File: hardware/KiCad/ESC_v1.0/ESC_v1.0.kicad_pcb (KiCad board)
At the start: 2 copper layers, 108 parts, among them J3 Conn_ARM_SWD_TagConnect_TC203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, Q1 NVMFS5C604N, Q2 NVMFS5C604N, Q3 NVMFS5C604N, Q4 NVMFS5C604N, Q5 NVMFS5C604N, Q6 NVMFS5C604N, U1 STM32G484CEU6, U2 LM5160A, U3 TPS7B92033, U4 2EDL8024, U5 2EDL8024, U6 2EDL8024, X1 16MHz

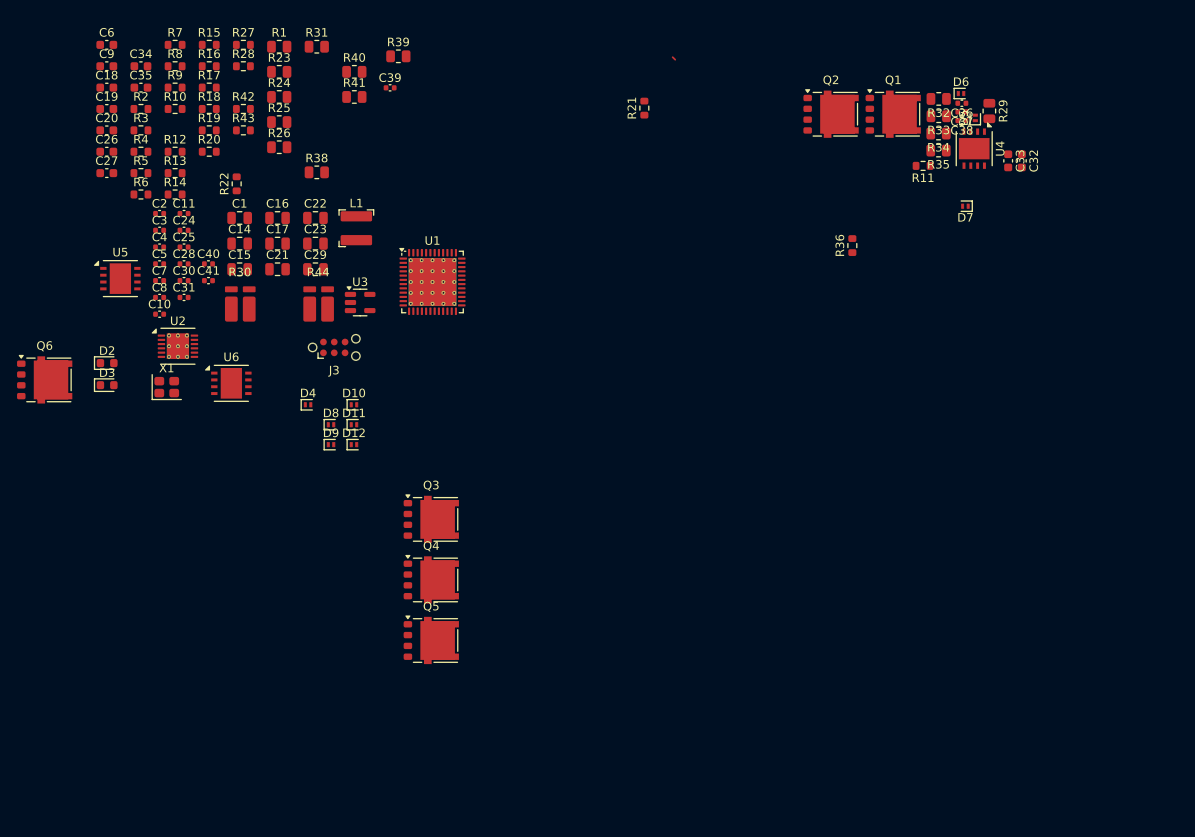
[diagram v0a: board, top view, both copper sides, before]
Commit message: Kicad
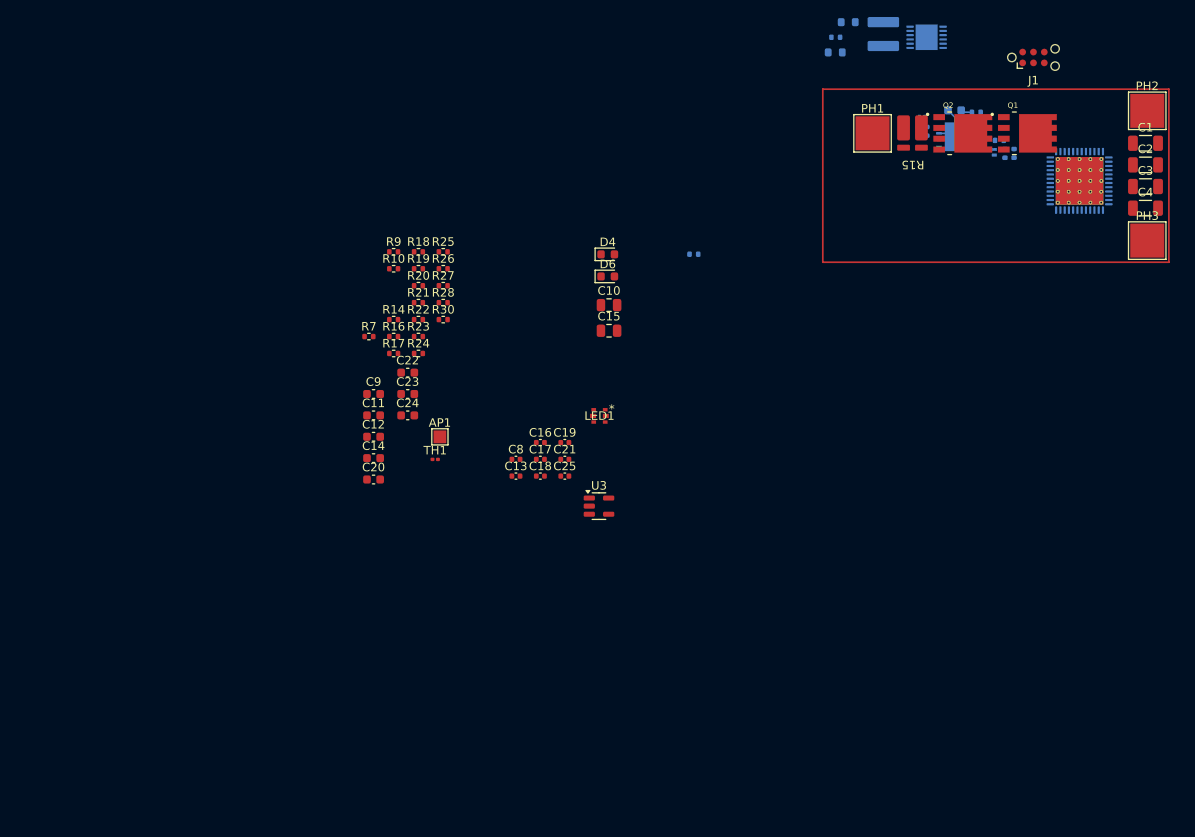
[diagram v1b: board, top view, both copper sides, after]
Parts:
- removed C26, C27, C32, C33, C34, C35: 1u, Capacitor_SMD:C_0603_1608Metric
- removed C28, C30, C31, C36, C37, C38, C39, C40, C41, C7: 100n, Capacitor_SMD:C_0402_1005Metric
- removed C29: 4.7u, Capacitor_SMD:C_0805_2012Metric
- removed D10, D11, D12, D7, D8, D9: RB161QS-40T18R, ESC-FootprintLib:Rohm_SMD1006
- removed J3: Conn_ARM_SWD_TagConnect_TC2030-NL, Connector:Tag-Connect_TC2030-IDC-NL_2x03_P1.27mm_Vertical
- removed Q3, Q4, Q5, Q6: NVMFS5C604N, ESC-FootprintLib:Onsemi_DFN5_DFNW5
- removed R29, R31: 5.1, Resistor_SMD:R_0805_2012Metric
- removed R32, R33, R34, R35, R38, R39, R40, R41: 10, Resistor_SMD:R_0805_2012Metric
- removed R36, R42, R43: 10k, Resistor_SMD:R_0603_1608Metric
- removed R44: 0.5, ESC-FootprintLib:Kelvin Shunt 1216 (3038)
- removed U5, U6: 2EDL8024, Package_DFN_QFN:DFN-8-1EP_4x4mm_P0.8mm_EP2.5x3.6mm
- removed X1: 16MHz, Crystal:Crystal_SMD_2520-4Pin_2.5x2.0mm
- added AP1: ActionPad, TestPoint:TestPoint_Pad_1.5x1.5mm, F.Cu at (68.1, 63.7)
- added C12: 1u, Capacitor_SMD:C_0603_1608Metric, F.Cu at (60.3, 63.7)
- added C13: 10n, Capacitor_SMD:C_0402_1005Metric, F.Cu at (77.0, 68.3)
- added J1: Conn_ARM_SWD_TagConnect_TC2030-NL, Connector:Tag-Connect_TC2030-IDC-NL_2x03_P1.27mm_Vertical, F.Cu at (137.8, 19.1)
- added LED1: 19-337C/RSBHGHC-A88/4T, ESC-FootprintLib:SMD-B_19-337C_EVE, F.Cu at (86.8, 61.2)
- added PH1: ~, TestPoint:TestPoint_Pad_4.0x4.0mm, F.Cu at (118.9, 28.0)
- added PH2: ~, TestPoint:TestPoint_Pad_4.0x4.0mm, F.Cu at (151.1, 25.4)
- added PH3: ~, TestPoint:TestPoint_Pad_4.0x4.0mm, F.Cu at (151.1, 40.6)
- added TH1: Thermistor_NTC, Resistor_SMD:R_0201_0603Metric, F.Cu at (67.5, 66.3)
- C1: value 4.7u -> 2.2u; footprint Capacitor_SMD:C_0805_2012Metric -> Capacitor_SMD:C_1206_3216Metric
- C10: value 10p -> 4.7u; footprint Capacitor_SMD:C_0402_1005Metric -> Capacitor_SMD:C_0805_2012Metric
- C11: value 10p -> 1u; footprint Capacitor_SMD:C_0402_1005Metric -> Capacitor_SMD:C_0603_1608Metric
- C14: value 22u -> 1u; footprint Capacitor_SMD:C_0805_2012Metric -> Capacitor_SMD:C_0603_1608Metric
- C15: value 22u -> 4.7u
- C16, C17: value 22u -> 100n; footprint Capacitor_SMD:C_0805_2012Metric -> Capacitor_SMD:C_0402_1005Metric
- C18, C19: value 1u -> 100n; footprint Capacitor_SMD:C_0603_1608Metric -> Capacitor_SMD:C_0402_1005Metric
- C2, C3, C4: value 100n -> 2.2u; footprint Capacitor_SMD:C_0402_1005Metric -> Capacitor_SMD:C_1206_3216Metric
- C21: value 100p -> 100n; footprint Capacitor_SMD:C_0805_2012Metric -> Capacitor_SMD:C_0402_1005Metric
- C22, C23: footprint Capacitor_SMD:C_0805_2012Metric -> Capacitor_SMD:C_0603_1608Metric
- C24: value 100n -> 100p; footprint Capacitor_SMD:C_0402_1005Metric -> Capacitor_SMD:C_0603_1608Metric
- C25: value 10n -> 100n
- C5: value 10n -> 1u; footprint Capacitor_SMD:C_0402_1005Metric -> Capacitor_SMD:C_0603_1608Metric; moved to B.Cu
- C6: value 1u -> 220n; footprint Capacitor_SMD:C_0603_1608Metric -> Capacitor_SMD:C_0402_1005Metric; moved to B.Cu
- C8: value 100n -> 10n
- D2, D3: value KT-0603W -> RB161QS-40T18R; footprint LED_SMD:LED_0603_1608Metric -> ESC-FootprintLib:Rohm_SMD1006; moved to B.Cu
- D4, D6: value RB161QS-40T18R -> KT-0603W; footprint ESC-FootprintLib:Rohm_SMD1006 -> LED_SMD:LED_0603_1608Metric
- D5, L1, R5: moved to B.Cu
- Q1, Q2: value NVMFS5C604N -> CSD18540Q5B; footprint ESC-FootprintLib:Onsemi_DFN5_DFNW5 -> ESC-FootprintLib:TRANS_CSD18540Q5B
- R1: value 5.1 -> 3.3; footprint Resistor_SMD:R_0805_2012Metric -> Resistor_SMD:R_0402_1005Metric; moved to B.Cu
- R10: value 47 -> 1k; footprint Resistor_SMD:R_0603_1608Metric -> Resistor_SMD:R_0402_1005Metric
- R11: value 10k -> 10; footprint Resistor_SMD:R_0603_1608Metric -> Resistor_SMD:R_0402_1005Metric; moved to B.Cu
- R12: value 47 -> 22k; moved to B.Cu
- R13: value 390 -> 10k; footprint Resistor_SMD:R_0603_1608Metric -> Resistor_SMD:R_0402_1005Metric; moved to B.Cu
- R14: value 390 -> 12k; footprint Resistor_SMD:R_0603_1608Metric -> Resistor_SMD:R_0402_1005Metric
- R15: value 5.6k -> 0.5; footprint Resistor_SMD:R_0603_1608Metric -> ESC-FootprintLib:Kelvin Shunt 1216 (3038)
- R16, R17: value 150 -> 10k; footprint Resistor_SMD:R_0603_1608Metric -> Resistor_SMD:R_0402_1005Metric
- R18: value 150 -> 100; footprint Resistor_SMD:R_0603_1608Metric -> Resistor_SMD:R_0402_1005Metric
- R19, R27, R28: value 10k -> 100; footprint Resistor_SMD:R_0603_1608Metric -> Resistor_SMD:R_0402_1005Metric
- R2: value 390 -> 10; footprint Resistor_SMD:R_0603_1608Metric -> Resistor_SMD:R_0402_1005Metric; moved to B.Cu
- R20: value 39k -> 200k; footprint Resistor_SMD:R_0603_1608Metric -> Resistor_SMD:R_0402_1005Metric
- R21: value 1k -> 33; footprint Resistor_SMD:R_0603_1608Metric -> Resistor_SMD:R_0402_1005Metric
- R22: value 120k -> 33; footprint Resistor_SMD:R_0603_1608Metric -> Resistor_SMD:R_0402_1005Metric
- R23, R25, R26: value 10 -> 1k; footprint Resistor_SMD:R_0805_2012Metric -> Resistor_SMD:R_0402_1005Metric
- R24: value 10 -> 33; footprint Resistor_SMD:R_0805_2012Metric -> Resistor_SMD:R_0402_1005Metric
- R3: value 22k -> 3.3; footprint Resistor_SMD:R_0603_1608Metric -> Resistor_SMD:R_0402_1005Metric; moved to B.Cu
- R30: value 0.5 -> 10k; footprint ESC-FootprintLib:Kelvin Shunt 1216 (3038) -> Resistor_SMD:R_0402_1005Metric
- R4: value 200k -> 10k; footprint Resistor_SMD:R_0603_1608Metric -> Resistor_SMD:R_0402_1005Metric; moved to B.Cu
- R6: value 5.6k -> 200k; footprint Resistor_SMD:R_0603_1608Metric -> Resistor_SMD:R_0402_1005Metric; moved to B.Cu
- R7: value 5.6k -> 100; footprint Resistor_SMD:R_0603_1608Metric -> Resistor_SMD:R_0402_1005Metric
- R8: value 390 -> 3.3; footprint Resistor_SMD:R_0603_1608Metric -> Resistor_SMD:R_0402_1005Metric; moved to B.Cu
- R9: value 47 -> 51k; footprint Resistor_SMD:R_0603_1608Metric -> Resistor_SMD:R_0402_1005Metric
- U1: value STM32G484CEU6 -> 2EDL8024; footprint Package_DFN_QFN:QFN-48-1EP_7x7mm_P0.5mm_EP5.6x5.6mm_ThermalVias -> ESC-FootprintLib:2EDL8x2x_PG-VDSON-8-4; moved to B.Cu
- U2: footprint Package_SON:WSON-12-1EP_4x4mm_P0.5mm_EP2.6x3mm_ThermalVias -> Package_SON:WSON-12-1EP_4x4mm_P0.5mm_EP2.6x3mm; moved to B.Cu
- U4: value 2EDL8024 -> STM32G484CEU6; footprint Package_DFN_QFN:DFN-8-1EP_4x4mm_P0.8mm_EP2.5x3.6mm -> Package_DFN_QFN:QFN-48-1EP_7x7mm_P0.5mm_EP5.6x5.6mm_ThermalVias; moved to B.Cu
- moved C2 115.9 mm to (150.9, 31.8)
- moved C3 115.9 mm to (150.9, 34.3)
- moved C4 115.9 mm to (150.9, 36.8)
- moved D3 107.7 mm to (133.2, 30.3), turned to -90 degrees
- moved D2 106.8 mm to (132.0, 27.0), turned to 90 degrees
- moved C1 106.7 mm to (150.9, 29.2)
- moved C6 103.6 mm to (132.0, 28.8), turned to -90 degrees
- moved R4 102.5 mm to (135.5, 30.4), turned to -90 degrees
- moved R2 101.6 mm to (134.4, 30.4), turned to 90 degrees
- moved U2 95.1 mm to (125.2, 16.8), turned to 180 degrees
- moved C5 95.1 mm to (128.5, 25.3), turned to 180 degrees
- moved R8 94.2 mm to (131.1, 25.6)
- moved R3 92.3 mm to (125.2, 27.8), turned to -90 degrees
- moved R1 85.3 mm to (133.8, 28.9)
- moved R15 84.5 mm to (124.6, 29.7), turned to 180 degrees
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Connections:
- C1 pad 1: +3V3 -> VM
- C1 pad 2: AGND -> PGND
- C10 pad 1: /HSE_OUT -> +3V3
- C10 pad 2: AGND -> GND
- C11 pad 1: /HSE_IN -> Net-(U2-SS)
- C11 pad 2: AGND -> GND
- C14 pad 1: VM -> +3V3A
- C14 pad 2: PGND -> AGND
- C15 pad 1: VM -> +3V3
- C15 pad 2: PGND -> GND
- C16 pad 1: VM -> +3V3
- C16 pad 2: PGND -> GND
- C17 pad 1: VM -> +3V3
- C17 pad 2: PGND -> GND
- C18 pad 1: +10V -> +3V3
- C18 pad 2: AGND -> GND
- C19 pad 1: Net-(U2-SS) -> +3V3REF
- C2 pad 1: +3V3 -> VM
- C2 pad 2: AGND -> PGND
- C20 pad 1: Net-(U2-FPWM) -> +3V3REF
- C21 pad 1: Net-(C21-Pad1) -> +3.3V
- C21 pad 2: AGND -> GND
- C22 pad 1: Net-(C22-Pad1) -> VSENSE1
- C22 pad 2: AGND -> GND
- C23 pad 1: Net-(C23-Pad1) -> VSENSE2
- C23 pad 2: AGND -> GND
- C24 pad 1: +3.3V -> VSENSE3
- C24 pad 2: AGND -> GND
- C25 pad 1: +10VNoise -> DEBUG_NRST
- C25 pad 2: Net-(U2-BST) -> GND
- C3 pad 1: +3V3 -> VM
- C3 pad 2: AGND -> PGND
- C4 pad 1: +3V3 -> VM
- C4 pad 2: AGND -> PGND
- C5 pad 1: +3V3A -> +10V
- C5 pad 2: AGND -> GND
- C6 pad 1: +3V3A -> /HB1
- C6 pad 2: AGND -> PH1
- C8 pad 1: DEBUG_NRST -> +10.5VNoise
- C8 pad 2: AGND -> Net-(U2-BST)
- C9 pad 1: +3V3REF -> +10.5V
- C9 pad 2: AGND -> GND
- D2 pad 1: AGND -> /HB1
- D3 pad 1: AGND -> /HO
- D4 pad 1: Net-(D4-K) -> GND
- D5 pad 1: /HB1 -> /LO
- D6 pad 1: /HO1 -> GND
- L1 pad 1: +10VNoise -> +10.5VNoise
- L1 pad 2: +10V -> +10.5V
- R1 pad 1: +10V -> /HO
- R1 pad 2: Net-(D4-A) -> Net-(Q1-G)
- R10 pad 1: VSENSE2 -> +10.5V
- R10 pad 2: Net-(C22-Pad1) -> Net-(D6-A)
- R11 pad 1: Net-(Q2-G) -> Net-(D5-A)
- R11 pad 2: AGND -> Net-(Q2-G)
- R12 pad 1: VSENSE3 -> Net-(U2-EN/UVLO)
- R12 pad 2: Net-(C23-Pad1) -> GND
- R13 pad 1: VSENSE2 -> Net-(Q2-G)
- R13 pad 2: AGND -> GND
- R14 pad 1: VSENSE1 -> Net-(U2-FB)
- R14 pad 2: AGND -> GND
- R15 pad 1: PH3 -> ISENSE1
- R15 pad 2: VSENSE3 -> GPH1
- R16 pad 1: +3V3 -> Net-(R16-Pad1)
- R16 pad 2: Net-(D3-A) -> PH1
- R17 pad 1: RGB_LED_G -> Net-(R17-Pad1)
- R17 pad 2: /LED_G_K -> PH2
- R18 pad 1: RGB_LED_B -> RGB_LED_G
- R18 pad 2: /LED_B_K -> /LED_G_K
- R19 pad 1: Net-(U2-FB) -> RGB_LED_B
- R19 pad 2: AGND -> /LED_B_K
- R2 pad 1: RGB_LED_R -> Net-(D3-A)
- R2 pad 2: /LED_R_K -> Net-(Q1-G)
- R20 pad 1: +10V -> /BOOT0
- R20 pad 2: Net-(U2-FB) -> GND
- R21 pad 1: +10V -> Net-(R17-Pad1)
- R21 pad 2: Net-(D2-A) -> VSENSE2
- R22 pad 1: /BOOT0 -> Net-(R16-Pad1)
- R22 pad 2: AGND -> VSENSE3
- R23 pad 1: Net-(D8-A) -> Net-(R17-Pad1)
- R23 pad 2: Net-(Q3-G) -> GND
- R24 pad 1: Net-(D8-K) -> Net-(R24-Pad1)
- R24 pad 2: Net-(Q3-G) -> VSENSE1
- R25 pad 1: Net-(D9-K) -> Net-(R24-Pad1)
- R25 pad 2: Net-(Q4-G) -> GND
- R26 pad 1: Net-(D9-A) -> Net-(R16-Pad1)
- R26 pad 2: Net-(Q4-G) -> GND
- R27 pad 1: Net-(Q3-G) -> /LED_R_K
- R27 pad 2: PH1 -> Net-(R27-Pad2)
- R28 pad 1: Net-(Q4-G) -> RGB_LED_R
- R28 pad 2: AGND -> Net-(R27-Pad2)
- R3 pad 1: Net-(U2-EN/UVLO) -> /LO
- R3 pad 2: AGND -> Net-(Q2-G)
- R30 pad 1: ISENSE1 -> Net-(R24-Pad1)
- R30 pad 2: AGND -> PH3
- R4 pad 1: VM -> Net-(Q1-G)
- R4 pad 2: Net-(U2-EN/UVLO) -> PH1
- R6 pad 1: PH2 -> VM
- R6 pad 2: VSENSE2 -> Net-(U2-EN/UVLO)
- R7 pad 1: PH1 -> +3V3
- R7 pad 2: VSENSE1 -> Net-(D4-A)
- R8 pad 1: VSENSE3 -> +10V
- R8 pad 2: AGND -> Net-(D2-A)
- R9 pad 1: VSENSE1 -> +10.5V
- R9 pad 2: Net-(C21-Pad1) -> Net-(U2-FB)
- U1 pad 1: +3V3 -> +10V
- U1 pad 2: unconnected-(U1-PC13-Pad2) -> /HB1
- U1 pad 3: unconnected-(U1-PC14-OSC32_IN-Pad3) -> /HO
- U1 pad 4: unconnected-(U1-PC15-OSC32_OUT-Pad4) -> PH1
- U1 pad 5: /HSE_IN -> PWM1
- U1 pad 6: /HSE_OUT -> PWM1N
- U1 pad 7: DEBUG_NRST -> GND
- U1 pad 8: unconnected-(U1-PA0-Pad8) -> /LO
- U2 pad 11: +10VNoise -> +10.5VNoise
- U2 pad 12: +10VNoise -> +10.5VNoise
- U2 pad 2: AGND -> GND
- U3 pad 1: +10V -> +10.5V
- U3 pad 2: AGND -> GND
- U3 pad 3: AGND -> GND
- U3 pad 4: AGND -> GND
- U4 pad 1: +10V -> +3V3
- U4 pad 2: /HB1 -> unconnected-(U4-PC13-Pad2)
- U4 pad 3: /HO1 -> unconnected-(U4-PC14-OSC32_IN-Pad3)
- U4 pad 4: PH1 -> unconnected-(U4-PC15-OSC32_OUT-Pad4)
- U4 pad 5: PWM1 -> /HSE_IN
- U4 pad 6: PWM1N -> /HSE_OUT
- U4 pad 7: AGND -> DEBUG_NRST
- U4 pad 8: /LO1 -> unconnected-(U4-PA0-Pad8)
- U4 pad 9: (no net) -> Net-(J2-Pin_2)
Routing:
- net GND: track 0.00 -> 5.53 mm
- net /HB1: track 0.00 -> 4.52 mm
- net +10V: track 0.00 -> 3.07 mm
- net PH1: track 0.00 -> 1.65 mm
- net Net-(D2-A): track 0.00 -> 1.27 mm

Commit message: V1 schematic
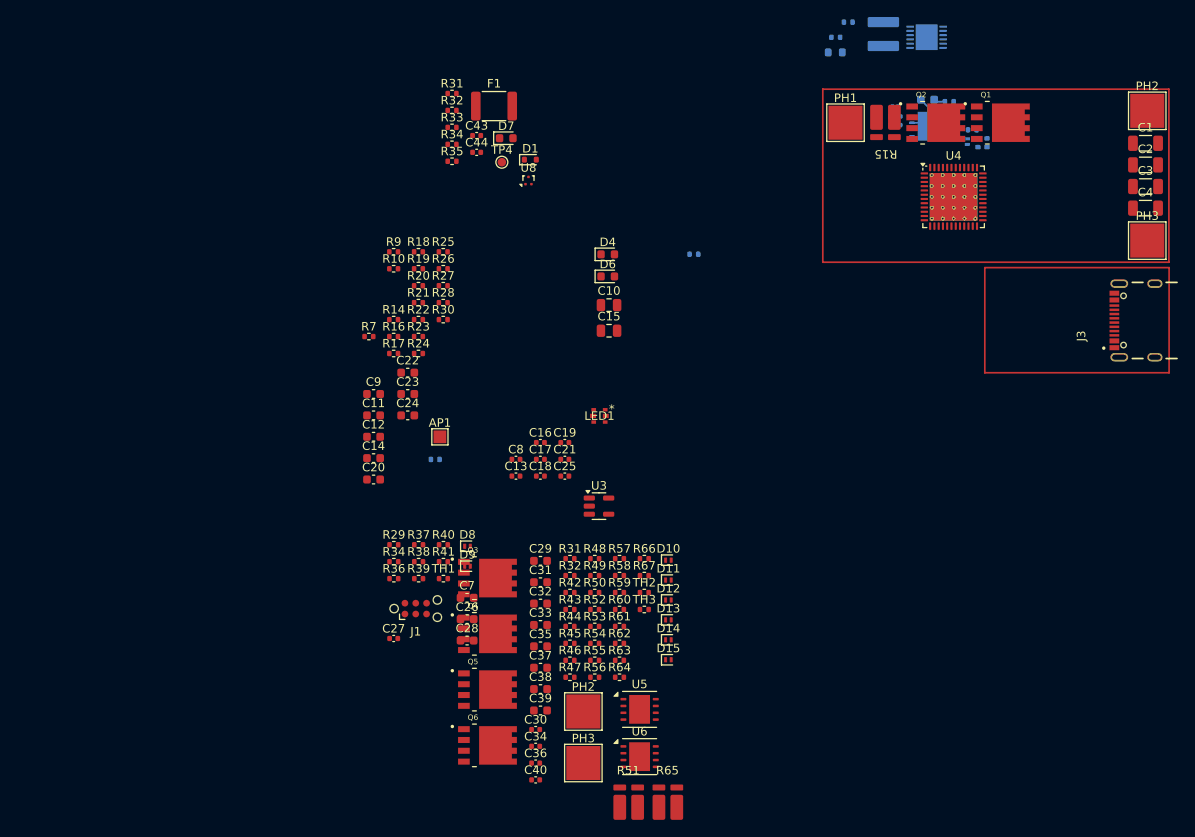
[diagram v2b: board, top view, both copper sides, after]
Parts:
- added C26: 100p, Capacitor_SMD:C_0603_1608Metric, F.Cu at (71.3, 85.1)
- added C27: 100n, Capacitor_SMD:C_0402_1005Metric, F.Cu at (62.6, 87.4)
- added C28: 100p, Capacitor_SMD:C_0603_1608Metric, F.Cu at (71.3, 87.6)
- added C29: 100p, Capacitor_SMD:C_0603_1608Metric, F.Cu at (79.9, 78.2)
- added C30: 220n, Capacitor_SMD:C_0402_1005Metric, F.Cu at (79.3, 98.1)
- added C31: 1u, Capacitor_SMD:C_0603_1608Metric, F.Cu at (79.9, 80.8)
- added C32: 100p, Capacitor_SMD:C_0603_1608Metric, F.Cu at (79.9, 83.3)
- added C33: 100p, Capacitor_SMD:C_0603_1608Metric, F.Cu at (79.9, 85.8)
- added C34: 100n, Capacitor_SMD:C_0402_1005Metric, F.Cu at (79.3, 100.0)
- added C35: 100p, Capacitor_SMD:C_0603_1608Metric, F.Cu at (79.9, 88.3)
- added C36: 220n, Capacitor_SMD:C_0402_1005Metric, F.Cu at (79.3, 102.0)
- added C37: 1u, Capacitor_SMD:C_0603_1608Metric, F.Cu at (79.9, 90.8)
- added C38: 100p, Capacitor_SMD:C_0603_1608Metric, F.Cu at (79.9, 93.3)
- added C39: 100p, Capacitor_SMD:C_0603_1608Metric, F.Cu at (79.9, 95.8)
- added C40: 100n, Capacitor_SMD:C_0402_1005Metric, F.Cu at (79.3, 104.0)
- added C43: 1u, Capacitor_SMD:C_0402_1005Metric, F.Cu at (72.4, 28.3)
- added C44: 100n, Capacitor_SMD:C_0402_1005Metric, F.Cu at (72.4, 30.3)
- added C7: 100p, Capacitor_SMD:C_0603_1608Metric, F.Cu at (71.3, 82.6)
- added D1: ESD5Zxx, Diode_SMD:D_SOD-523, F.Cu at (78.7, 31.1)
- added D10: RB161QS-40T18R, ESC-FootprintLib:Rohm_SMD1006, F.Cu at (94.9, 78.2)
- added D11: RB161QS-40T18R, ESC-FootprintLib:Rohm_SMD1006, F.Cu at (94.9, 80.5)
- added D12: RB161QS-40T18R, ESC-FootprintLib:Rohm_SMD1006, F.Cu at (94.9, 82.8)
- added D13: RB161QS-40T18R, ESC-FootprintLib:Rohm_SMD1006, F.Cu at (94.9, 85.2)
- added D14: RB161QS-40T18R, ESC-FootprintLib:Rohm_SMD1006, F.Cu at (94.9, 87.5)
- added D15: RB161QS-40T18R, ESC-FootprintLib:Rohm_SMD1006, F.Cu at (94.9, 89.9)
- added D7: LED, LED_SMD:LED_0603_1608Metric, F.Cu at (75.9, 28.6)
- added D8: RB161QS-40T18R, ESC-FootprintLib:Rohm_SMD1006, F.Cu at (71.3, 76.5)
- added D9: RB161QS-40T18R, ESC-FootprintLib:Rohm_SMD1006, F.Cu at (71.3, 78.9)
- added F1: Polyfuse, Resistor_SMD:R_1812_4532Metric, F.Cu at (74.4, 24.8)
- added J3: USB4105-GF-A, ESC-FootprintLib:GCT_USB4105-GF-A, F.Cu at (152.0, 50.0)
- added PH2: ~, TestPoint:TestPoint_Pad_4.0x4.0mm, F.Cu at (84.9, 95.9)
- added PH3: ~, TestPoint:TestPoint_Pad_4.0x4.0mm, F.Cu at (84.9, 102.0)
- added Q3: CSD18540Q5B, ESC-FootprintLib:TRANS_CSD18540Q5B, F.Cu at (73.7, 80.3)
- added Q4: CSD18540Q5B, ESC-FootprintLib:TRANS_CSD18540Q5B, F.Cu at (73.7, 86.8)
- added Q5: CSD18540Q5B, ESC-FootprintLib:TRANS_CSD18540Q5B, F.Cu at (73.7, 93.4)
- added Q6: CSD18540Q5B, ESC-FootprintLib:TRANS_CSD18540Q5B, F.Cu at (73.7, 99.9)
- added R29: 33, Resistor_SMD:R_0402_1005Metric, F.Cu at (62.7, 76.4)
- added R31: 3.3, Resistor_SMD:R_0402_1005Metric, F.Cu at (69.5, 23.4)
- added R31: 3.3, Resistor_SMD:R_0402_1005Metric, F.Cu at (83.3, 78.0)
- added R32: 10, Resistor_SMD:R_0402_1005Metric, F.Cu at (83.3, 80.0)
- added R32: 10, Resistor_SMD:R_0402_1005Metric, F.Cu at (69.5, 25.4)
- added R33: 220, Resistor_SMD:R_0402_1005Metric, F.Cu at (69.5, 27.3)
- added R34: 5.1k, Resistor_SMD:R_0402_1005Metric, F.Cu at (62.7, 78.3)
- added R34: 5.1k, Resistor_SMD:R_0402_1005Metric, F.Cu at (69.5, 29.3)
- added R35: 5.1k, Resistor_SMD:R_0402_1005Metric, F.Cu at (69.5, 31.3)
- added R36: 10k, Resistor_SMD:R_0402_1005Metric, F.Cu at (62.7, 80.3)
- added R37: 200k, Resistor_SMD:R_0402_1005Metric, F.Cu at (65.6, 76.4)
- added R38: 1k, Resistor_SMD:R_0402_1005Metric, F.Cu at (65.6, 78.3)
- added R39: 33, Resistor_SMD:R_0402_1005Metric, F.Cu at (65.6, 80.3)
- added R40: 10k, Resistor_SMD:R_0402_1005Metric, F.Cu at (68.5, 76.4)
- added R41: 10k, Resistor_SMD:R_0402_1005Metric, F.Cu at (68.5, 78.3)
- added R42: 3.3, Resistor_SMD:R_0402_1005Metric, F.Cu at (83.3, 82.0)
- added R43: 33, Resistor_SMD:R_0402_1005Metric, F.Cu at (83.3, 84.0)
- added R44: 10k, Resistor_SMD:R_0402_1005Metric, F.Cu at (83.3, 85.9)
- added R45: 10k, Resistor_SMD:R_0402_1005Metric, F.Cu at (83.3, 87.9)
- added R46: 1k, Resistor_SMD:R_0402_1005Metric, F.Cu at (83.3, 89.9)
- added R47: 3.3, Resistor_SMD:R_0402_1005Metric, F.Cu at (83.3, 91.9)
- added R48: 10, Resistor_SMD:R_0402_1005Metric, F.Cu at (86.2, 78.0)
- added R49: 200k, Resistor_SMD:R_0402_1005Metric, F.Cu at (86.2, 80.0)
- added R50: 10k, Resistor_SMD:R_0402_1005Metric, F.Cu at (86.2, 82.0)
- added R51: 0.5m, ESC-FootprintLib:Kelvin Shunt 1216 (3038), F.Cu at (89.2, 104.9)
- added R52: 33, Resistor_SMD:R_0402_1005Metric, F.Cu at (86.2, 84.0)
- added R53: 10k, Resistor_SMD:R_0402_1005Metric, F.Cu at (86.2, 85.9)
- added R54: 3.3, Resistor_SMD:R_0402_1005Metric, F.Cu at (86.2, 87.9)
- added R55: 10, Resistor_SMD:R_0402_1005Metric, F.Cu at (86.2, 89.9)
- added R56: 3.3, Resistor_SMD:R_0402_1005Metric, F.Cu at (86.2, 91.9)
- added R57: 33, Resistor_SMD:R_0402_1005Metric, F.Cu at (89.2, 78.0)
- added R58: 10k, Resistor_SMD:R_0402_1005Metric, F.Cu at (89.2, 80.0)
- added R59: 10k, Resistor_SMD:R_0402_1005Metric, F.Cu at (89.2, 82.0)
- added R60: 1k, Resistor_SMD:R_0402_1005Metric, F.Cu at (89.2, 84.0)
- added R61: 3.3, Resistor_SMD:R_0402_1005Metric, F.Cu at (89.2, 85.9)
- added R62: 10, Resistor_SMD:R_0402_1005Metric, F.Cu at (89.2, 87.9)
- added R63: 200k, Resistor_SMD:R_0402_1005Metric, F.Cu at (89.2, 89.9)
- added R64: 10k, Resistor_SMD:R_0402_1005Metric, F.Cu at (89.2, 91.9)
- added R65: 0.5m, ESC-FootprintLib:Kelvin Shunt 1216 (3038), F.Cu at (93.8, 104.9)
- added R66: 33, Resistor_SMD:R_0402_1005Metric, F.Cu at (92.1, 78.0)
- added R67: 10k, Resistor_SMD:R_0402_1005Metric, F.Cu at (92.1, 80.0)
- added TH1: Thermistor_NTC, Resistor_SMD:R_0402_1005Metric, F.Cu at (68.5, 80.3)
- added TH2: Thermistor_NTC, Resistor_SMD:R_0402_1005Metric, F.Cu at (92.1, 82.0)
- added TH3: Thermistor_NTC, Resistor_SMD:R_0402_1005Metric, F.Cu at (92.1, 84.0)
- added TP4: TestPoint, TestPoint:TestPoint_Pad_D1.0mm, F.Cu at (75.3, 31.4)
- added U5: 2EDL8024, ESC-FootprintLib:2EDL8x2x_PG-VDSON-8-4, F.Cu at (91.5, 95.7)
- added U6: 2EDL8024, ESC-FootprintLib:2EDL8x2x_PG-VDSON-8-4, F.Cu at (91.5, 101.2)
- added U8: TPD2EUSB30A, Package_TO_SOT_SMD:Texas_DRT-3, F.Cu at (78.5, 33.6)
- R12: footprint Resistor_SMD:R_0603_1608Metric -> Resistor_SMD:R_0402_1005Metric
- R15: value 0.5 -> 0.5m
- TH1: footprint Resistor_SMD:R_0201_0603Metric -> Resistor_SMD:R_0402_1005Metric; moved to B.Cu
- U4: moved to F.Cu
- moved J1 97.2 mm to (65.2, 83.9)
- moved U4 14.9 mm to (128.4, 35.5), turned to 0 degrees
- moved R8 3.41 mm to (127.9, 24.3)
- moved U1 3.41 mm to (125.4, 27.2)
- moved D3 3.41 mm to (130.0, 29.0)
- moved Q1 3.41 mm to (133.9, 26.8)
- moved C5 3.41 mm to (125.3, 24.1)
- moved R11 3.41 mm to (121.0, 26.6)
- moved R15 3.41 mm to (121.4, 28.5)
- moved D5 3.41 mm to (121.5, 24.9)
- moved PH1 3.41 mm to (115.7, 26.8)
- moved Q2 3.41 mm to (126.3, 26.8)
- moved R3 3.41 mm to (122.1, 26.6)
- moved R4 3.41 mm to (132.3, 29.2)
- moved C6 3.41 mm to (128.8, 27.6)
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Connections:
- AP1 pad 1: /BOOT0 -> Net-(AP1-Pad1)
- C1 pad 2: PGND -> GND
- C2 pad 2: PGND -> GND
- C3 pad 2: PGND -> GND
- C4 pad 2: PGND -> GND
- C9 pad 1: +10.5V -> Net-(D8-K)
- PH2 pad 1: VM -> PH2
- PH3 pad 1: PGND -> PH3
- Q2 pad 3: ISENSE1 -> +ISENS1
- R15 pad 1: ISENSE1 -> +ISENS1
- R15 pad 2: GPH1 -> Net-(NT3-Pad2)
- R20 pad 1: /BOOT0 -> Net-(AP1-Pad1)
- TH1 pad 1: GPH1 -> +ISENS1
- TH1 pad 2: unconnected-(TH1-Pad2) -> Net-(R29-Pad2)
- U2 pad 1: AGND -> GND
- U3 pad 1: +10.5V -> Net-(D8-K)
- U4 pad 15: unconnected-(U4-PA7-Pad15) -> +ISENS2
- U4 pad 18: unconnected-(U4-PB1-Pad18) -> +VSENS1
- U4 pad 2: unconnected-(U4-PC13-Pad2) -> RGB_LED_B
- U4 pad 22: unconnected-(U4-PB10-Pad22) -> PWM2N
- U4 pad 25: unconnected-(U4-PB12-Pad25) -> +VSENS2
- U4 pad 26: unconnected-(U4-PB13-Pad26) -> +TSENS2
- U4 pad 27: unconnected-(U4-PB14-Pad27) -> +ISENS3
- U4 pad 28: unconnected-(U4-PB15-Pad28) -> +TSENS3
- U4 pad 29: unconnected-(U4-PC6-Pad29) -> PWM1
- U4 pad 3: unconnected-(U4-PC14-OSC32_IN-Pad3) -> RGB_LED_G
- U4 pad 30: unconnected-(U4-PA8-Pad30) -> +VSENS3
- U4 pad 32: unconnected-(U4-PA10-Pad32) -> PWM/DSHOOT
- U4 pad 33: unconnected-(U4-PA11-Pad33) -> USB_D-
- U4 pad 34: unconnected-(U4-PA12-Pad34) -> USB_D+
- U4 pad 38: unconnected-(U4-PA15-Pad38) -> VBAT
- U4 pad 39: unconnected-(U4-PC10-Pad39) -> PWM1N
- U4 pad 4: unconnected-(U4-PC15-OSC32_OUT-Pad4) -> RGB_LED_R
- U4 pad 43: unconnected-(U4-PB5-Pad43) -> PWM3N
- U4 pad 46: /BOOT0 -> PWM2
- U4 pad 47: unconnected-(U4-PB9-Pad47) -> PWM3
- U4 pad 5: /HSE_IN -> unconnected-(U4-PF0-OSC_IN-Pad5)
- U4 pad 6: /HSE_OUT -> unconnected-(U4-PF1-OSC_OUT-Pad6)
- U4 pad 8: unconnected-(U4-PA0-Pad8) -> +TSENS1
- U4 pad 9: Net-(J2-Pin_2) -> +ISENS1
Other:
- copper layers 2 -> 6
